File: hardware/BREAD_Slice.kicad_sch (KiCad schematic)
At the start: 15 parts, among them J1 Conn_01x10_Female, J2 I2C_01x04

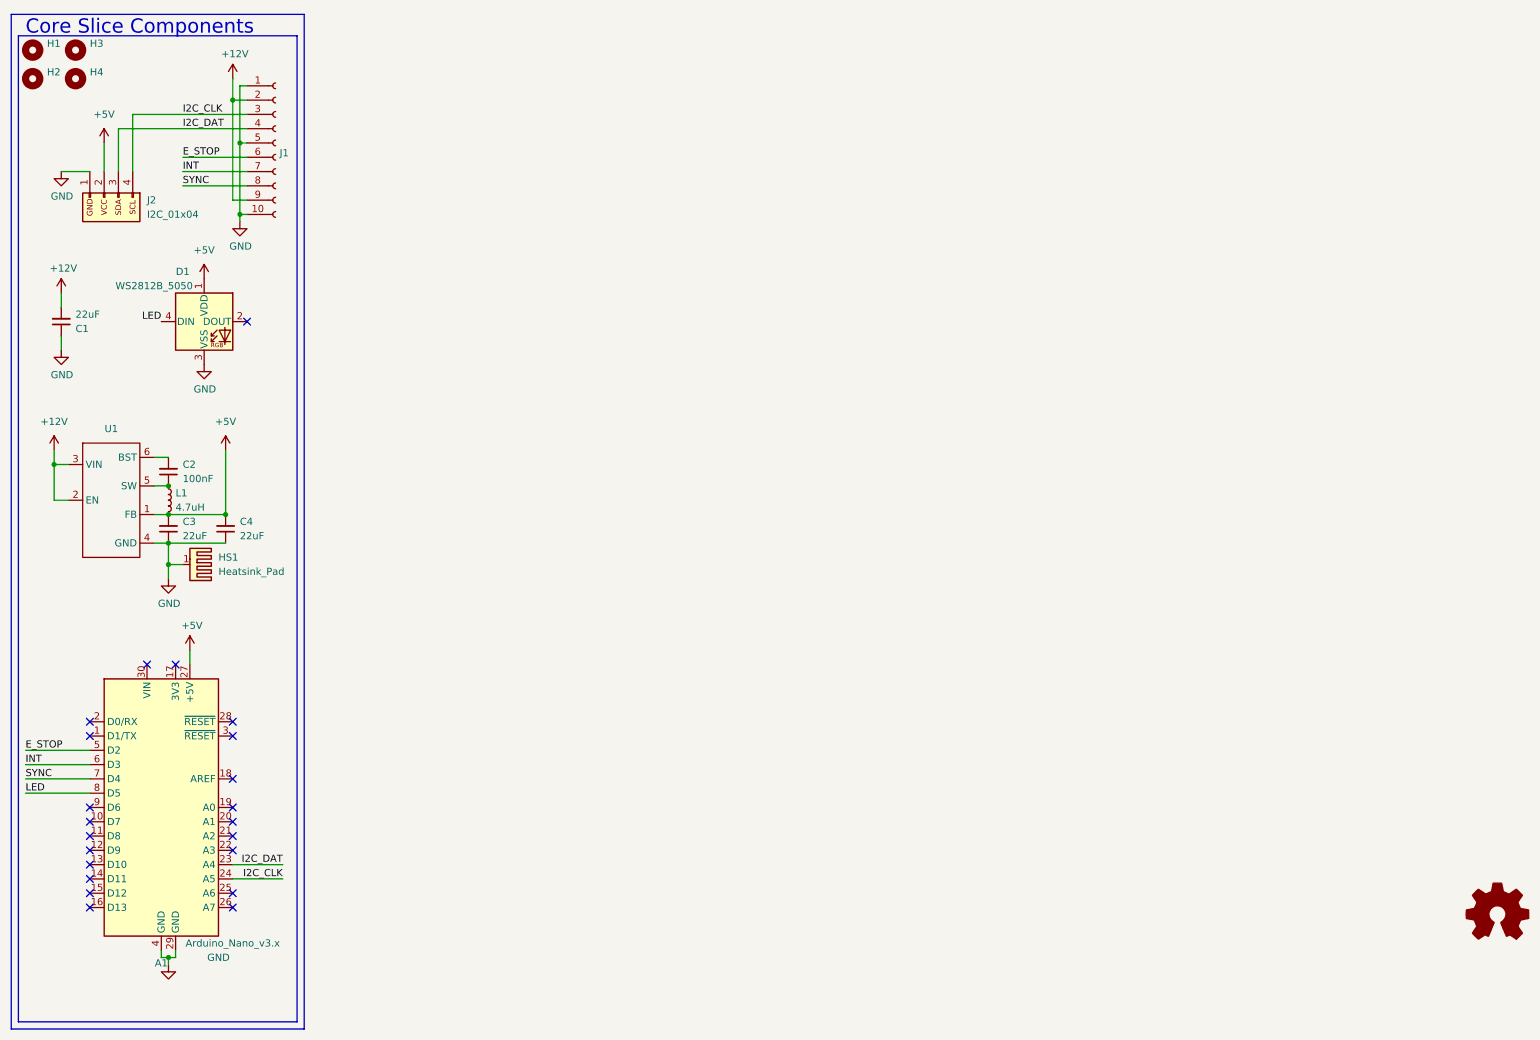
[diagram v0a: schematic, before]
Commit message: Initial commit
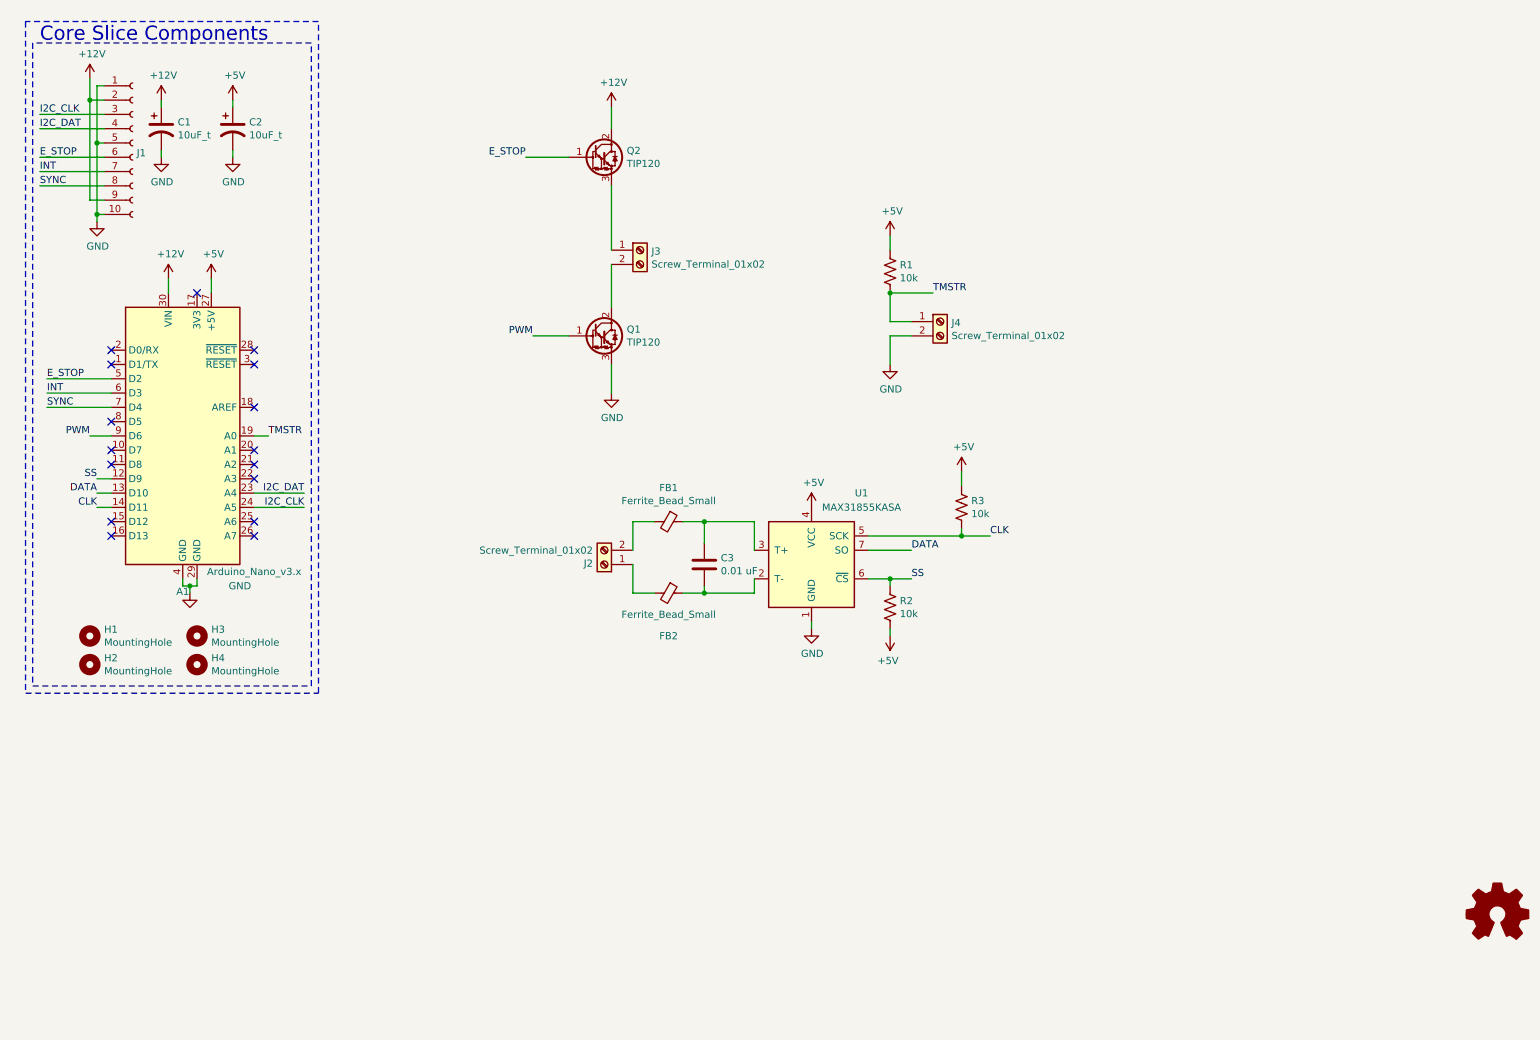
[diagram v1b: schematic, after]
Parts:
- removed C1, C3, C4: 22uF, Capacitor_SMD:C_1206_3216Metric, symbol Device:C_Small
- removed C2: 100nF, Capacitor_SMD:C_1206_3216Metric, symbol Device:C_Small
- removed D1: WS2812B_5050, SparkFun-LED:WS2812-5050-4PIN, symbol SparkFun-LED:WS2812B_5050
- removed HS1: Heatsink_Pad, SparkFun-Fuse:Thermal Pad, symbol Mechanical:Heatsink_Pad
- removed J2: I2C_01x04, Connector_JST:JST_SH_SM04B-SRSS-TB_1x04-1MP_P1.00mm_Horizontal, symbol SparkFun-Connector:I2C_01x04
- removed L1: 4.7uH, Inductor_SMD:L_1210_3225Metric, symbol Device:L_Small
- removed U1: ~, Package_TO_SOT_SMD:TSOT-23-6, symbol SparkFun-DiscreteSemi:AP63205
- added C1, C2: 10uF_t, OCI_UPL_FOOTPRINTS:C_2312, symbol BREAD_Slice-rescue:10uF_t-OCI_UPL_2_Capacitors
- added C3: 0.01 uF, OCI_UPL_FOOTPRINTS:C_1206_HandSoldering, symbol Device:C
- added FB1, FB2: Ferrite_Bead_Small, OCI_UPL_FOOTPRINTS:R_1206_HandSoldering, symbol BREAD_Slice-rescue:Ferrite_Bead_Small-Device
- added J2, J3, J4: Screw_Terminal_01x02, OCI_UPL_FOOTPRINTS:TerminalBlock_Pheonix_MKDS1.5-2pol, symbol Connector:Screw_Terminal_01x02
- added Logo1: Logo_Open_Hardware_Small, Symbol:OSHW-Symbol_6.7x6mm_SilkScreen, symbol Graphic:Logo_Open_Hardware_Small
- added Q1, Q2: TIP120, Package_TO_SOT_THT:TO-220-3_Vertical, symbol Transistor_BJT:TIP120
- added R1, R2, R3: 10k, OCI_UPL_FOOTPRINTS:R_1206_HandSoldering, symbol Device:R_US
- added U1: MAX31855KASA, Package_SO:SOIC-8_3.9x4.9mm_P1.27mm, symbol BREAD_Slice-rescue:MAX31855KASA-Sensor_Temperature
- H1, H4: footprint MountingHole:MountingHole_5mm -> MountingHole:MountingHole_3.2mm_M3_DIN965_Pad
- H2: renamed from H3; footprint MountingHole:MountingHole_5mm -> MountingHole:MountingHole_3.2mm_M3_DIN965_Pad
- H3: renamed from H2; footprint MountingHole:MountingHole_5mm -> MountingHole:MountingHole_3.2mm_M3_DIN965_Pad
- J1: symbol Connector:Conn_01x10_Female -> BREAD_Slice-rescue:Conn_01x10_Female-Connector
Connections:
- net +12V: now also A1.30 (VIN), C1.1, Q2.2 (C)
- net +5V: now also C2.1, R1.1, R2.2, R3.1, U1.4 (VCC)
- net E_STOP: now also Q2.1 (B)
- net GND: now also C1.2, C2.2, J4.2 (Pin_2), Q1.3 (E), U1.1 (GND)
- net SS: now reaches A1.12 (D9)
- net SS: now also R2.1, U1.6 (~{CS})
- net DATA: now reaches A1.13 (D10)
- net DATA: now also U1.7 (SO)
- net CLK: now reaches A1.14 (D11)
- net CLK: now also R3.2, U1.5 (SCK)
- net TMSTR: now reaches A1.19 (A0)
- net TMSTR: now also J4.1 (Pin_1), R1.2
- net PWM: now reaches A1.9 (D6)
- net PWM: now also Q1.1 (B)
- net LED: no longer names the net of A1.8 (D5)
- new net: J3.2 (Pin_2), Q1.2 (C)
- new net: J3.1 (Pin_1), Q2.3 (E)
- new net: FB2.2, J2.1 (Pin_1)
- new net: FB1.2, J2.2 (Pin_2)
- new net: C3.1, FB1.1, U1.3 (T+)
- new net: C3.2, FB2.1, U1.2 (T-)
- no-connect marks 22 -> 16
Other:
- moved on the sheet: A1, H1, H2, H3, H4, J1
